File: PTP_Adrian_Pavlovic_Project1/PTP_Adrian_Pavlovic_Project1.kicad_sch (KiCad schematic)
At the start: 25 parts, among them J1 Screw_Terminal_01x02, SW1 SW_Push, SW2 SW_SPDT_312, U1 LM2574N-5, U6 74LVC1G11, U7 NE555P

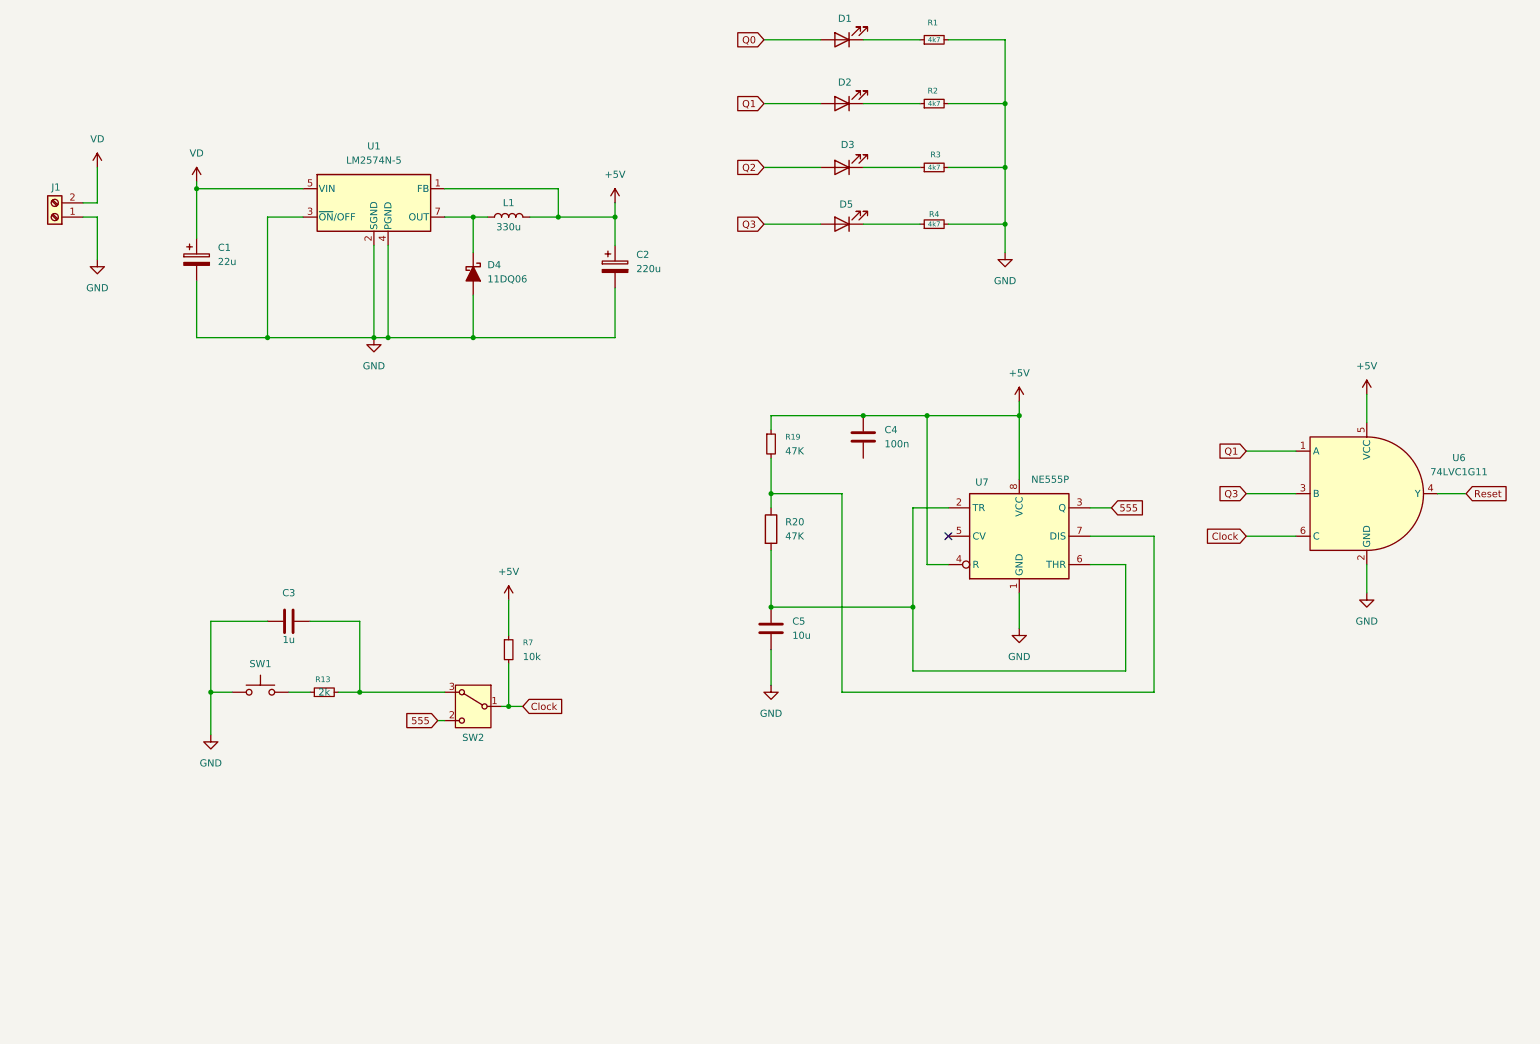
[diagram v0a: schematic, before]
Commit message: project1
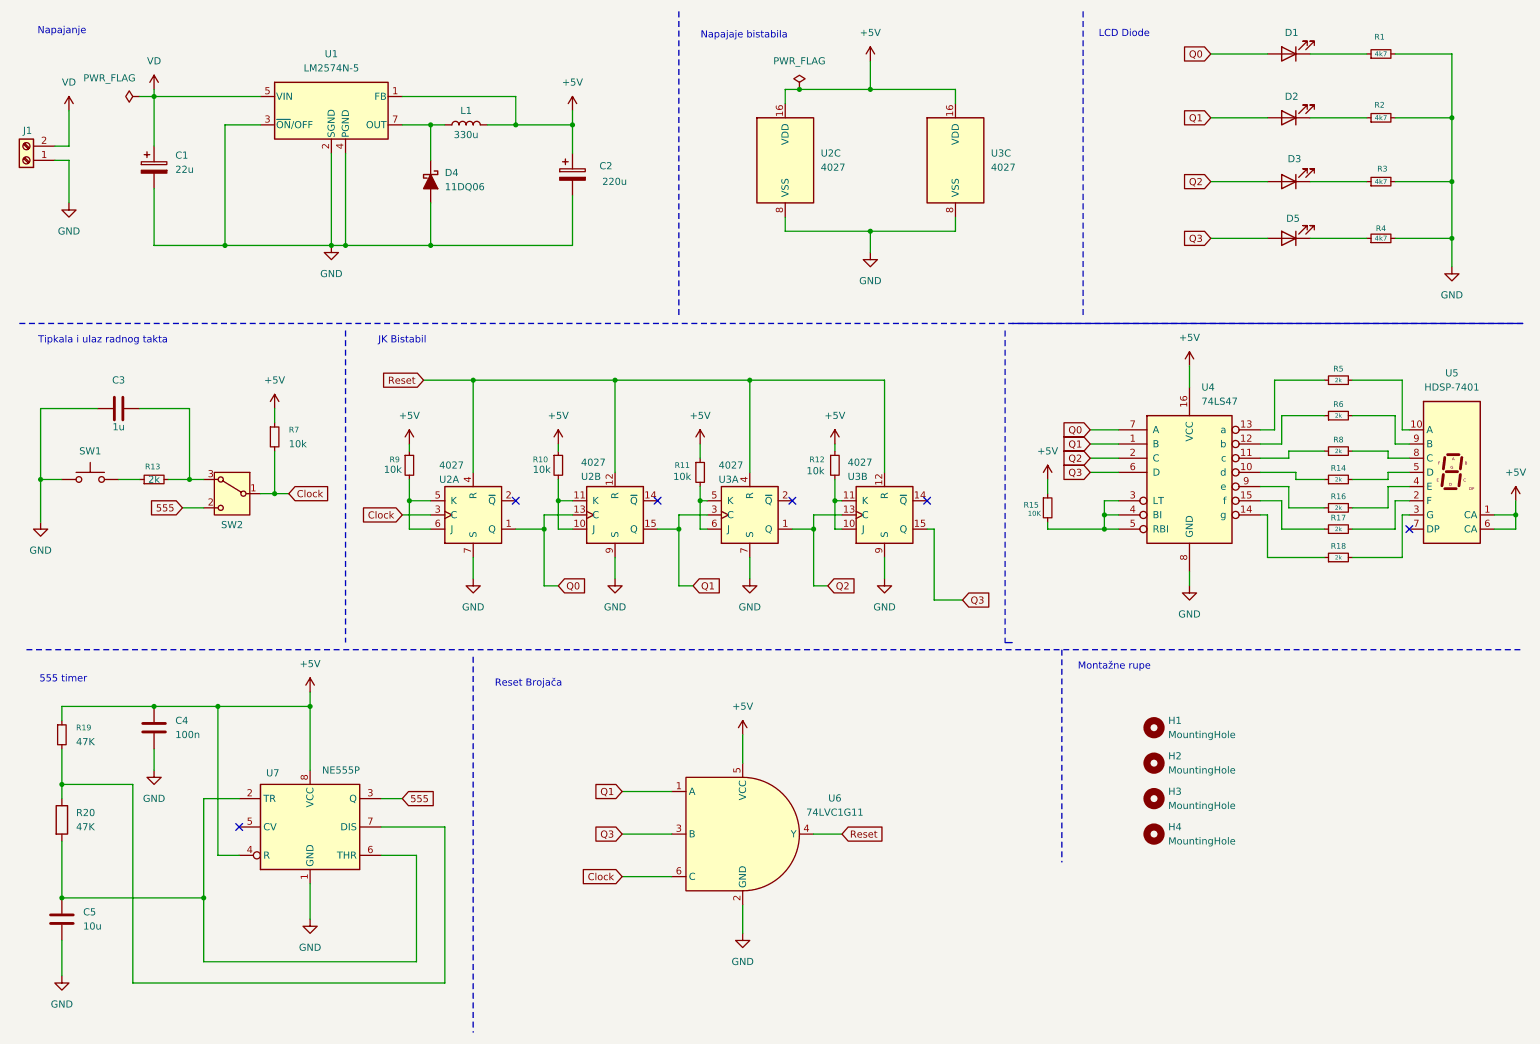
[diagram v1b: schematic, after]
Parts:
- added H1, H2, H3, H4: MountingHole, symbol Mechanical:MountingHole
- added R10, R11, R12, R9: 10k, symbol Device:R_Small
- added R14, R16, R17, R18, R5, R6, R8: 2k, symbol Device:R_Small
- added R15: 10K, symbol Device:R_Small
- added U2, U3: 4027, symbol 4xxx:4027
- added U4: 74LS47, symbol 74xx:74LS47
- added U5: HDSP-7401, Display_7Segment:HDSP-7401, symbol Display_Character:HDSP-7401
- C1: footprint (none) -> Capacitor_THT:CP_Radial_D5.0mm_P2.00mm; Manufacturer (none) -> AISHI; Manufacturer Part Number (none) -> EWH1EM220D11OT
- C2: footprint (none) -> Capacitor_THT:CP_Radial_D5.0mm_P2.00mm; Manufacturer (none) -> SAMWHA; Manufacturer Part Number (none) -> RD1A227M05011BB
- C3: footprint (none) -> Capacitor_SMD:C_1206_3216Metric_Pad1.33x1.80mm_HandSolder; Manufacturer (none) -> SAMSUNG; Manufacturer Part Number (none) -> CL31B105KBHNNNE
- C4: footprint (none) -> Capacitor_SMD:C_1206_3216Metric_Pad1.33x1.80mm_HandSolder; Manufacturer (none) -> SAMSUNG; Manufacturer Part Number (none) -> CL31B104KBCNNNC
- C5: footprint (none) -> Capacitor_SMD:C_1206_3216Metric_Pad1.33x1.80mm_HandSolder; Manufacturer (none) -> SAMSUNG; Manufacturer Part Number (none) -> CL31A106KBHNNNE
- U1: footprint Package_DIP:DIP-8_W7.62mm -> Package_DIP:DIP-8_W7.62mm_Socket_LongPads; Manufacture Part Number (none) -> LM2574N-5G; Manufacturer (none) -> ONSEMI
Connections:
- net +5V: now also R10.1, R11.1, R12.1, R15.1, R9.1, U2.16 (VDD), U3.16 (VDD), U4.16 (VCC), U5.1 (CA), U5.6 (CA)
- net Clock: now also U2.3 (C)
- net GND: now also C4.2, U2.7 (S), U2.8 (VSS), U2.9 (S), U3.7 (S), U3.8 (VSS), U3.9 (S), U4.8 (GND)
- net Q0: now also U2.1 (Q), U2.13 (C), U4.7 (A)
- net Q1: now also U2.15 (Q), U3.3 (C), U4.1 (B)
- net Q2: now also U3.1 (Q), U3.13 (C), U4.2 (C)
- net Q3: now also U3.15 (Q), U4.6 (D)
- net Reset: now also U2.12 (R), U2.4 (R), U3.12 (R), U3.4 (R)
- new net: R10.2, U2.10 (J), U2.11 (K)
- new net: R15.2, U4.3 (LT), U4.4 (BI), U4.5 (RBI)
- new net: R11.2, U3.5 (K), U3.6 (J)
- new net: R5.1, U4.13 (a)
- new net: R5.2, U5.10 (A)
- new net: R18.1, U4.14 (g)
- new net: R18.2, U5.3 (G)
- new net: R14.1, U4.10 (d)
- new net: R14.2, U5.5 (D)
- new net: R9.2, U2.5 (K), U2.6 (J)
- new net: R8.1, U4.11 (c)
- new net: R6.1, U4.12 (b)
- new net: R17.1, U4.15 (f)
- new net: R16.1, U4.9 (e)
- new net: R16.2, U5.4 (E)
- new net: R12.2, U3.10 (J), U3.11 (K)
- new net: R8.2, U5.8 (C)
- new net: R6.2, U5.9 (B)
- new net: R17.2, U5.2 (F)
- no-connect marks 1 -> 6
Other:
- note added: "555 timer"
- note added: "JK Bistabil"
- note added: "LCD Diode"
- note added: "Montažne rupe"
- note added: "Napajaje bistabila"
- note added: "Napajanje"
- note added: "Reset Brojača"
- note added: "Tipkala i ulaz radnog takta"
- moved on the sheet: C1, C2, C3, C4, C5, D1, D2, D3, D4, D5, J1, L1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

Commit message: Vjezba7
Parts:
- D1, D2, D3, D5: footprint (none) -> LED_THT:LED_D5.0mm
- D4: footprint (none) -> Diode_THT:D_DO-41_SOD81_P12.70mm_Horizontal
- H1, H2, H3, H4: footprint (none) -> MountingHole:MountingHole_5.5mm
- J1: footprint (none) -> TerminalBlock_MetzConnect:TerminalBlock_MetzConnect_Type011_RT05502HBLC_1x02_P5.00mm_Horizontal
- L1: footprint (none) -> Inductor_THT:L_Radial_D7.2mm_P3.00mm_Murata_1700
- R1, R2, R3, R4: footprint (none) -> Resistor_THT:R_Axial_DIN0207_L6.3mm_D2.5mm_P10.16mm_Horizontal
- R10, R11, R12, R13, R14, R15, R16, R17, R18, R19, R20, R5, R6, R7, R8, R9: footprint (none) -> Resistor_SMD:R_1206_3216Metric_Pad1.30x1.75mm_HandSolder
- SW1: footprint (none) -> Button_Switch_THT:SW_PUSH_6mm_H4.3mm
- SW2: footprint (none) -> Button_Switch_THT:SW_Slide_SPDT_Straight_CK_OS102011MS2Q
- U2, U3, U4: footprint (none) -> Package_DIP:DIP-16_W7.62mm_Socket_LongPads
- U6: footprint SOT-23-6:SOT-23-6 -> Package_TO_SOT_SMD:SOT-23-6
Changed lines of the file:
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@@
 			)
 		)
-		(property "Footprint" ""
+		(property "Footprint" "Resistor_THT:R_Axial_DIN0207_L6.3mm_D2.5mm_P10.16mm_Horizontal"
 			(at 257.81 53.34 0)
 			(effects
@@
 			)
 		)
-		(property "Footprint" ""
+		(property "Footprint" "MountingHole:MountingHole_5.5mm"
 			(at 217.17 147.32 0)
 			(effects
@@
 			)
 		)
-		(property "Footprint" ""
+		(property "Footprint" "LED_THT:LED_D5.0mm"
 			(at 241.3 20.32 0)
 			(effects
@@
 			)
 		)
-		(property "Footprint" ""
+		(property "Footprint" "Package_DIP:DIP-16_W7.62mm_Socket_LongPads"
 			(at 120.65 102.87 0)
 			(effects
@@
 			)
 		)
-		(property "Footprint" ""
+		(property "Footprint" "Resistor_THT:R_Axial_DIN0207_L6.3mm_D2.5mm_P10.16mm_Horizontal"
 			(at 257.81 31.75 0)
 			(effects
@@
 			)
 		)
-		(property "Footprint" ""
+		(property "Footprint" "Button_Switch_THT:SW_Slide_SPDT_Straight_CK_OS102011MS2Q"
 			(at 52.07 109.22 0)
 			(effects
@@
 			)
 		)
-		(property "Footprint" ""
+		(property "Footprint" "Resistor_SMD:R_1206_3216Metric_Pad1.30x1.75mm_HandSolder"
 			(at 198.12 101.6 0)
 			(effects
@@
 			)
 		)
-		(property "Footprint" ""
+		(property "Footprint" "Package_DIP:DIP-16_W7.62mm_Socket_LongPads"
 			(at 144.78 102.87 0)
 			(effects
@@
 			)
 		)
-		(property "Footprint" ""
+		(property "Footprint" "Resistor_SMD:R_1206_3216Metric_Pad1.30x1.75mm_HandSolder"
 			(at 21.59 142.24 0)
 			(effects
@@
 			)
 		)
-		(property "Footprint" ""
+		(property "Footprint" "MountingHole:MountingHole_5.5mm"
 			(at 217.17 160.02 0)
 			(effects
@@
 			)
 		)
-		(property "Footprint" ""
+		(property "Footprint" "MountingHole:MountingHole_5.5mm"
 			(at 217.17 153.67 0)
 			(effects
@@
 			)
 		)
-		(property "Footprint" ""
+		(property "Footprint" "Package_DIP:DIP-16_W7.62mm_Socket_LongPads"
 			(at 151.13 39.37 0)
 			(effects
@@
 			)
 		)
-		(property "Footprint" ""
+		(property "Footprint" "LED_THT:LED_D5.0mm"
 			(at 241.3 53.34 0)
 			(effects
@@
 			)
 		)
-		(property "Footprint" ""
+		(property "Footprint" "Resistor_SMD:R_1206_3216Metric_Pad1.30x1.75mm_HandSolder"
 			(at 250.19 78.74 0)
 			(effects
@@
 			)
 		)
-		(property "Footprint" ""
+		(property "Footprint" "Resistor_SMD:R_1206_3216Metric_Pad1.30x1.75mm_HandSolder"
 			(at 250.19 110.49 0)
 			(effects
@@
 			)
 		)
-		(property "Footprint" ""
+		(property "Footprint" "LED_THT:LED_D5.0mm"
 			(at 241.3 31.75 0)
 			(effects
@@
 			)
 		)
-		(property "Footprint" ""
+		(property "Footprint" "Resistor_SMD:R_1206_3216Metric_Pad1.30x1.75mm_HandSolder"
 			(at 250.19 96.52 0)
 			(effects
@@
 			)
 		)
-		(property "Footprint" ""
+		(property "Footprint" "Resistor_SMD:R_1206_3216Metric_Pad1.30x1.75mm_HandSolder"
 			(at 135.89 95.25 0)
 			(effects
@@
 			)
 		)
-		(property "Footprint" ""
+		(property "Footprint" "LED_THT:LED_D5.0mm"
 			(at 241.3 43.18 0)
 			(effects
@@
 			)
 		)
-		(property "Footprint" ""
+		(property "Footprint" "Package_DIP:DIP-16_W7.62mm_Socket_LongPads"
 			(at 95.25 102.87 0)
 			(effects
@@
 			)
 		)
-		(property "Footprint" ""
+		(property "Footprint" "Resistor_SMD:R_1206_3216Metric_Pad1.30x1.75mm_HandSolder"
 			(at 59.69 88.9 0)
 			(effects
@@
 			)
 		)
-		(property "Footprint" ""
+		(property "Footprint" "Resistor_THT:R_Axial_DIN0207_L6.3mm_D2.5mm_P10.16mm_Horizontal"
 			(at 257.81 43.18 0)
 			(effects
@@
 			)
 		)
-		(property "Footprint" ""
+		(property "Footprint" "Resistor_SMD:R_1206_3216Metric_Pad1.30x1.75mm_HandSolder"
 			(at 19.812 157.48 90)
 			(effects
@@
 			)
 		)
-		(property "Footprint" ""
+		(property "Footprint" "Resistor_SMD:R_1206_3216Metric_Pad1.30x1.75mm_HandSolder"
 			(at 110.49 93.98 0)
 			(effects
@@
 			)
 		)
-		(property "Footprint" ""
+		(property "Footprint" "Inductor_THT:L_Radial_D7.2mm_P3.00mm_Murata_1700"
 			(at 93.98 33.02 0)
 			(effects
@@
 			)
 		)
-		(property "Footprint" ""
+		(property "Footprint" "Package_DIP:DIP-16_W7.62mm_Socket_LongPads"
 			(at 223.52 95.25 0)
 			(effects
@@
 			)
 		)
-		(property "Footprint" ""
+		(property "Footprint" "Resistor_SMD:R_1206_3216Metric_Pad1.30x1.75mm_HandSolder"
 			(at 250.19 101.6 0)
 			(effects
@@
 			)
 		)
-		(property "Footprint" ""
+		(property "Footprint" "MountingHole:MountingHole_5.5mm"
 			(at 217.17 140.97 0)
 			(effects
@@
 			)
 		)
-		(property "Footprint" ""
+		(property "Footprint" "Button_Switch_THT:SW_PUSH_6mm_H4.3mm"
 			(at 26.67 91.44 0)
 			(effects
@@
 			)
 		)
-		(property "Footprint" ""
+		(property "Footprint" "Package_DIP:DIP-16_W7.62mm_Socket_LongPads"
 			(at 168.91 102.87 0)
 			(effects
@@
 			)
 		)
-		(property "Footprint" ""
+		(property "Footprint" "Package_DIP:DIP-16_W7.62mm_Socket_LongPads"
 			(at 181.61 39.37 0)
 			(effects
@@
 			)
 		)
-		(property "Footprint" ""
+		(property "Footprint" "TerminalBlock_MetzConnect:TerminalBlock_MetzConnect_Type011_RT05502HBLC_1x02_P5.00mm_Horizontal"
 			(at 15.24 39.37 0)
 			(effects
@@
 			)
 		)
-		(property "Footprint" ""
+		(property "Footprint" "Resistor_THT:R_Axial_DIN0207_L6.3mm_D2.5mm_P10.16mm_Horizontal"
 			(at 257.81 20.32 0)
 			(effects
@@
 			)
 		)
-		(property "Footprint" ""
+		(property "Footprint" "Resistor_SMD:R_1206_3216Metric_Pad1.30x1.75mm_HandSolder"
 			(at 38.1 96.52 0)
 			(effects
@@
 			)
 		)
-		(property "Footprint" ""
+		(property "Footprint" "Resistor_SMD:R_1206_3216Metric_Pad1.30x1.75mm_HandSolder"
 			(at 250.19 91.44 0)
 			(effects
@@
 			)
 		)
-		(property "Footprint" ""
+		(property "Footprint" "Resistor_SMD:R_1206_3216Metric_Pad1.30x1.75mm_HandSolder"
 			(at 83.82 93.98 0)
 			(effects
@@
 			)
 		)
-		(property "Footprint" ""
+		(property "Footprint" "Resistor_SMD:R_1206_3216Metric_Pad1.30x1.75mm_HandSolder"
 			(at 250.19 85.09 0)
 			(effects
@@
 			)
 		)
-		(property "Footprint" ""
+		(property "Footprint" "Diode_THT:D_DO-41_SOD81_P12.70mm_Horizontal"
 			(at 87.63 43.18 0)
 			(effects
@@
 			)
 		)
-		(property "Footprint" ""
+		(property "Footprint" "Resistor_SMD:R_1206_3216Metric_Pad1.30x1.75mm_HandSolder"
 			(at 250.19 105.41 0)
 			(effects
@@
 			)
 		)
-		(property "Footprint" "SOT-23-6:SOT-23-6"
+		(property "Footprint" "Package_TO_SOT_SMD:SOT-23-6"
 			(at 158.75 147.32 0)
 			(effects
@@
 			)
 		)
-		(property "Footprint" ""
+		(property "Footprint" "Resistor_SMD:R_1206_3216Metric_Pad1.30x1.75mm_HandSolder"
 			(at 160.02 93.98 0)
 			(effects

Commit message: Zadnja vježba
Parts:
- D4: Manufacturer (none) -> SMC DIODE SOLUTIONS
- J1: Manufacturer (none) -> DEGSON ELECTRONICS
- L1: Manufacturer (none) -> FERROCORE; Manufacturer Part Number (none) -> COIL0608-0.33
- R14, R16, R17, R18, R5, R6, R8: Manufacturer (none) -> ROYALOHM; Manufacturer Part Number (none) -> 1206S4F2001T5E
- R19, R20: Manufacturer (none) -> ROYALOHM; Manufacturer Part Number (none) -> 1206S4J0473T5E
- SW1: Manufacturer (none) -> microswitch TACT; Manufacturer Part Number (none) -> TACT-64N-F
- SW2: Manufacturer (none) -> C&K; Manufacturer Part Number (none) -> OS102011MS2QN1C
- U2, U3: Manufacturer (none) -> RENESAS; Manufacturer Part Number (none) -> CD4027BMS
- U4: Manufacturer (none) -> TEXAS INSTRUMENTS; Manufacturer Part Number (none) -> SN74LS47N
- U5: Manufacturer (none) -> FORYARD; Manufacturer Part Number (none) -> FYS-3911BUHR-21
- U6: Manufacturer (none) -> TEXAS INSTRUMENTS; Manufacturer Part Number (none) -> SN74LVC1G11DBVR
- U7: Manufacturer (none) -> TEXAS INSTRUMENTS; Manufacturer Part Number (none) -> NE555P
